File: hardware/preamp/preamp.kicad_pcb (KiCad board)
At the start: 2 copper layers, 45 x 17 mm, 32 parts, among them J1 I/O, J2 Conn 1, J3 Conn 2, Q1 2SC3324, Q2 2SC3324, U1 TLV170DBV

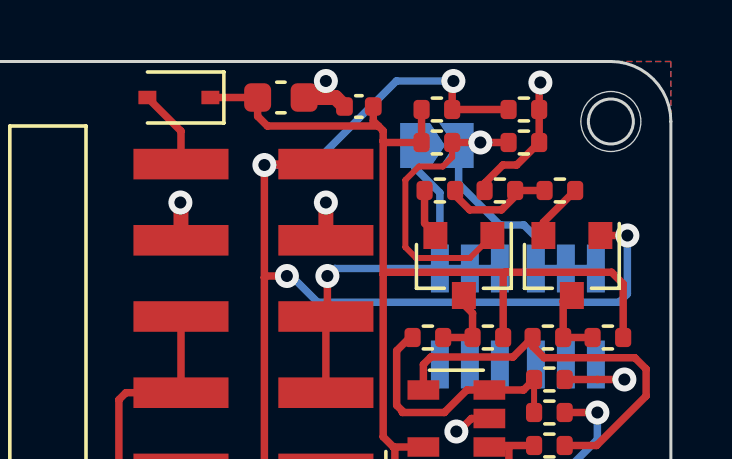
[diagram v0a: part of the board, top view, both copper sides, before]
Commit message: Passive board updates
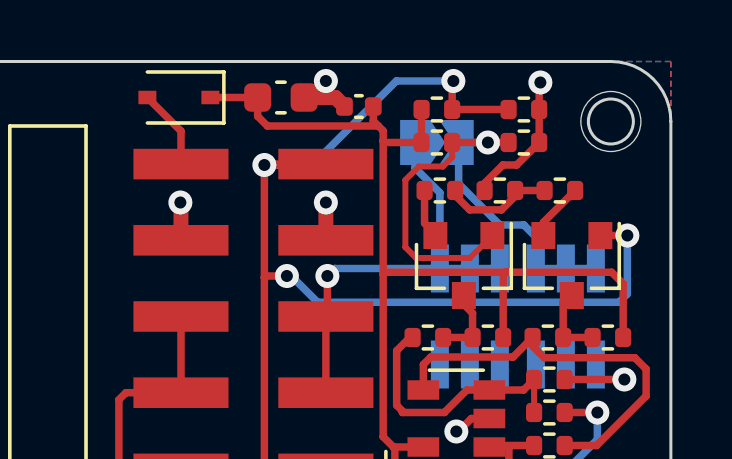
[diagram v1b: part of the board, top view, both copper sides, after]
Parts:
- moved JP1 0.10 mm to (142.2, 102.7)

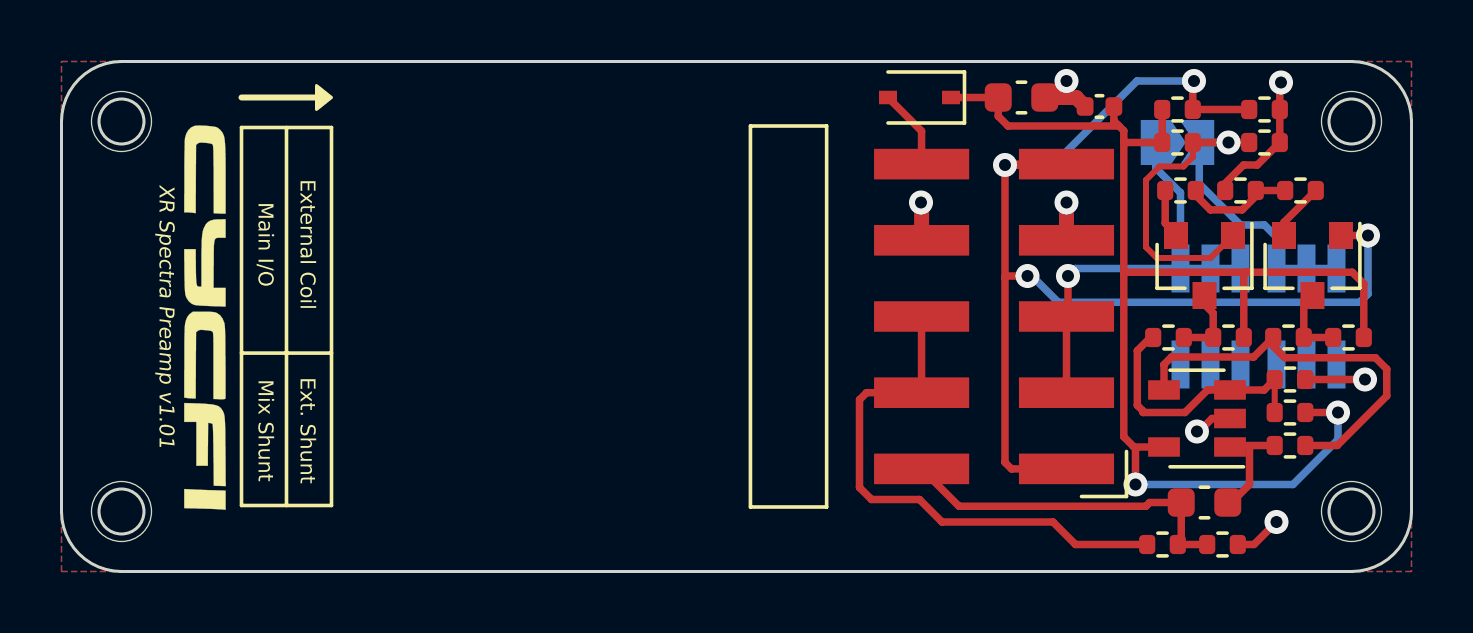
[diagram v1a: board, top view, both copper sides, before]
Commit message: updates for v1.01
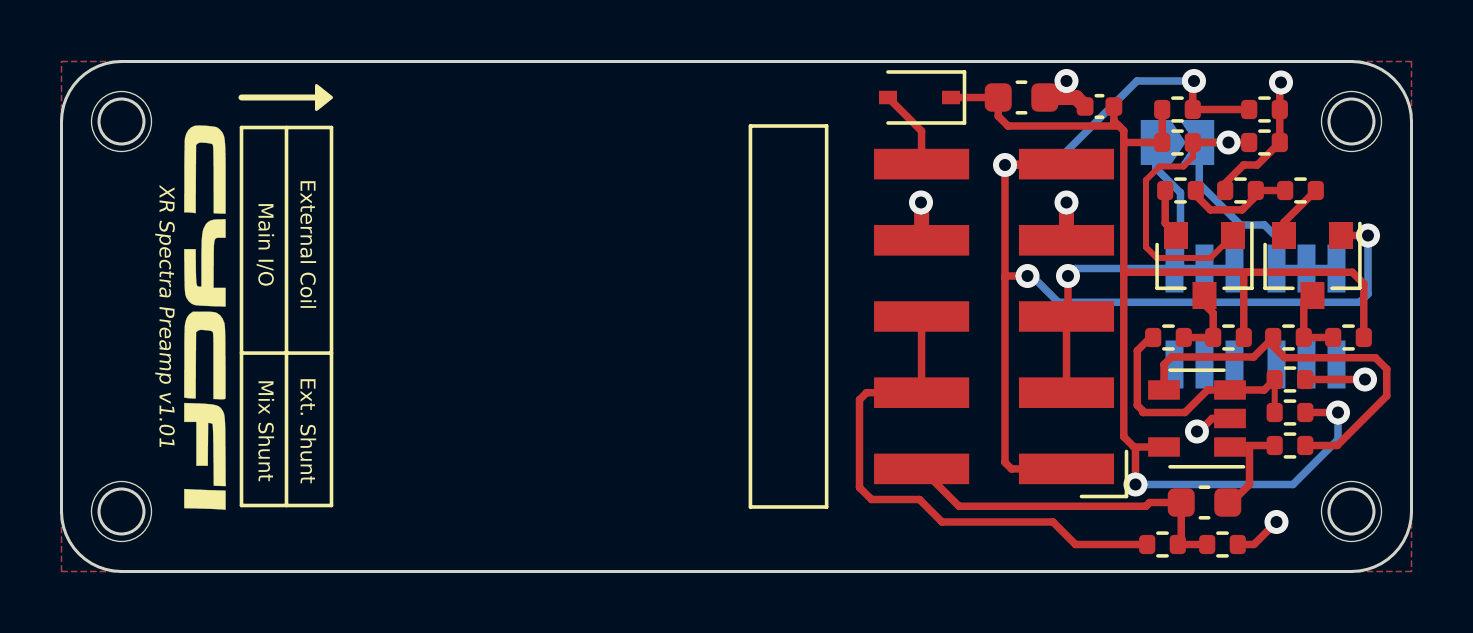
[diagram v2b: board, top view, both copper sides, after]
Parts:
- moved J2 0.20 mm to (143.1, 108.5)
